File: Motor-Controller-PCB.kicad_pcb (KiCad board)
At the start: 2 copper layers, 12 parts, among them Q1 AO3401A

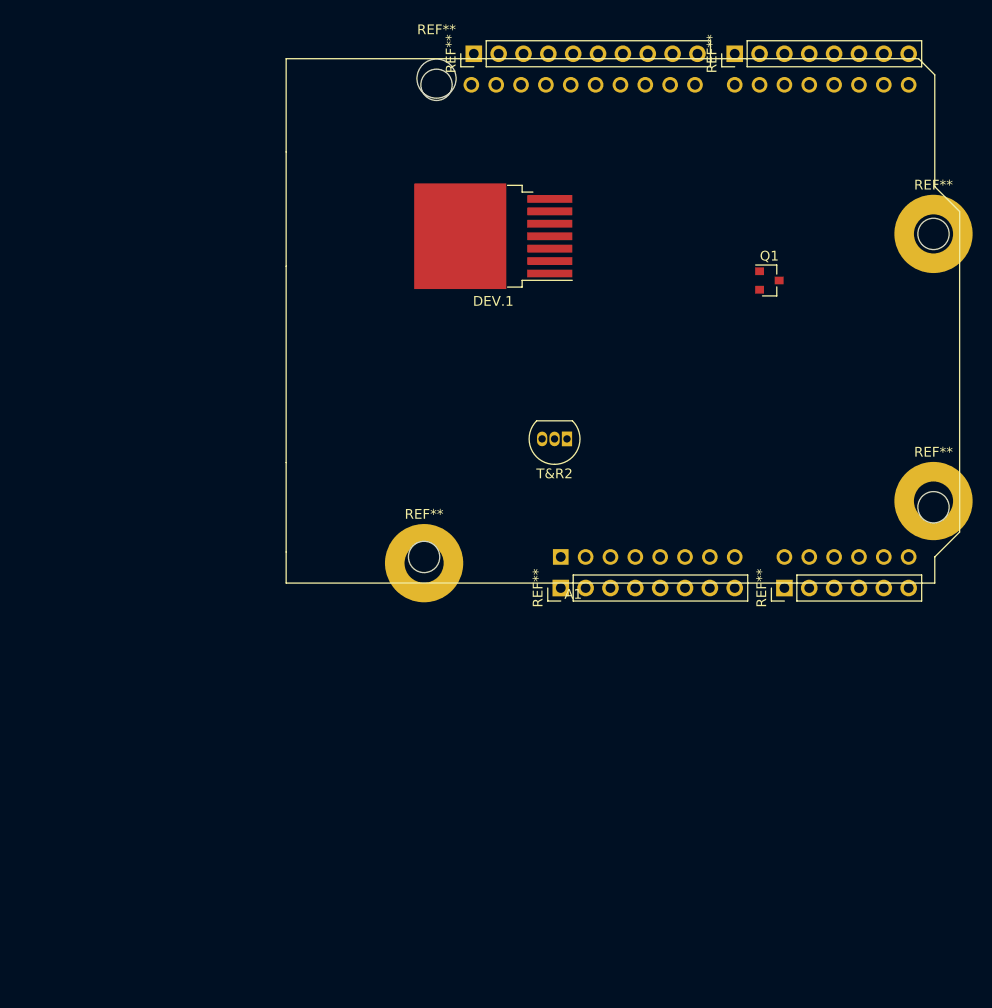
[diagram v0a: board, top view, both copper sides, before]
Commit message: layouting
almost done
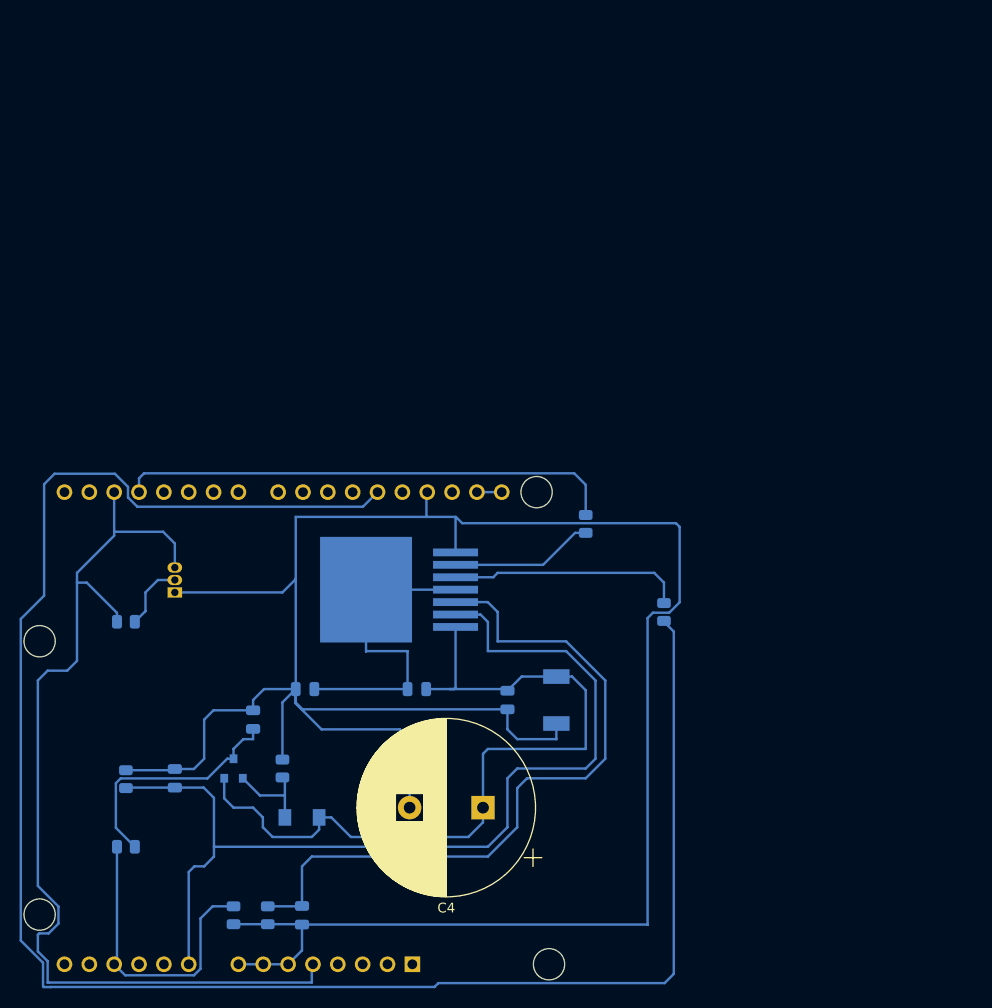
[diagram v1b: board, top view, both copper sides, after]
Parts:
- removed REF**: MountingHole_4mm, MountingHole:MountingHole_4mm
- removed REF** (x3): MountingHole_4mm_Pad, MountingHole:MountingHole_4mm_Pad
- removed REF**: PinHeader_1x06_P2.54mm_Vertical, Connector_PinHeader_2.54mm:PinHeader_1x06_P2.54mm_Vertical
- removed REF** (x2): PinHeader_1x08_P2.54mm_Vertical, Connector_PinHeader_2.54mm:PinHeader_1x08_P2.54mm_Vertical
- removed REF**: PinHeader_1x10_P2.54mm_Vertical, Connector_PinHeader_2.54mm:PinHeader_1x10_P2.54mm_Vertical
- added C10: 1nF, Capacitor_SMD:C_0805_2012Metric, B.Cu at (132.0, 102.0)
- added C11: 100nF, Capacitor_SMD:C_0805_2012Metric, B.Cu at (145.0, 116.0)
- added C12: 100uF, Capacitor_SMD:C_0805_2012Metric, B.Cu at (140.0, 96.0)
- added C14: 100nF, Capacitor_SMD:C_0805_2012Metric, B.Cu at (166.0, 94.0)
- added C4: 50V & 1500u, Capacitor_THT:CP_Radial_D18.0mm_P7.50mm, F.Cu at (163.5, 105.0)
- added C5: 220nF, Capacitor_SMD:C_0805_2012Metric, B.Cu at (145.3, 92.9)
- added C6: 220nF, Capacitor_SMD:C_0805_2012Metric, B.Cu at (156.7, 92.9)
- added D2: ZMY39, Diode_SMD:D_MELF, B.Cu at (171.0, 94.0)
- added D3: BZV55-C10, Diode_SMD:D_MiniMELF, B.Cu at (145.0, 106.0)
- added R1: 10K, Resistor_SMD:R_0805_2012Metric, B.Cu at (174.0, 76.0)
- added R12: 4.7K, Resistor_SMD:R_0805_2012Metric, B.Cu at (127.0, 86.0)
- added R13: 10K, Resistor_SMD:R_0805_2012Metric, B.Cu at (127.0, 109.0)
- added R14: 1K, Resistor_SMD:R_0805_2012Metric, B.Cu at (138.0, 116.0)
- added R15: 10K, Resistor_SMD:R_0805_2012Metric, B.Cu at (143.0, 101.0)
- added R5: 10K, Resistor_SMD:R_0805_2012Metric, B.Cu at (182.0, 85.0)
- added R7: 1K, Resistor_SMD:R_0805_2012Metric, B.Cu at (127.0, 102.1)
- added R9: 470, Resistor_SMD:R_0805_2012Metric, B.Cu at (141.5, 116.0)
- A1, DEV.1, Q1, T&R2: moved to B.Cu
- moved Q1 74.1 mm to (138.0, 101.0), turned to 90 degrees
- moved A1 58.2 mm to (184.2, 123.5), turned to 180 degrees
- moved T&R2 43.0 mm to (132.0, 83.0), turned to 90 degrees
- moved DEV.1 37.4 mm to (154.9, 82.7)
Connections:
- net Net-(C5-Pad2) renamed OUT_1
- DEV.1 pad 7: Net-(C1-Pad2) -> Net-(C14-Pad1)
- Q1 pad 2: GNDREF -> Net-(C14-Pad1)
- Q1 pad 3: VS -> VBAT
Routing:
- net GNDREF: track 0.00 -> 257.0 mm
- net Net-(A1-Pad27): track 0.00 -> 192.0 mm
- net 5V_ARDUINO: track 0.00 -> 101.6 mm
- net Net-(A1-Pad9): track 0.00 -> 100.6 mm
- net Net-(C14-Pad1): track 0.00 -> 81.8 mm
- net Net-(C11-Pad1): track 0.00 -> 73.8 mm
- net Net-(A1-Pad18): track 0.00 -> 50.9 mm
- net OUT_1: track 0.00 -> 33.1 mm
- net Net-(A1-Pad12): track 0.00 -> 30.7 mm
- net VBAT: track 0.00 -> 24.8 mm
- net Net-(DEV.1-Pad3): track 0.00 -> 24.0 mm
- net Net-(DEV.1-Pad2): track 0.00 -> 14.7 mm
- net Net-(D3-Pad2): track 0.00 -> 9.22 mm
- net Net-(R12-Pad1): track 0.00 -> 6.98 mm
- net Net-(A1-Pad31): track 0.00 -> 2.54 mm
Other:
- rule pad_to_mask_clearance: 0 -> 0.0508
- rule via_min_size: 0.4 -> 0.5
